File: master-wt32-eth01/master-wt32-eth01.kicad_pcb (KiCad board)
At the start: 2 copper layers, 61 x 72.4 mm, 12 parts, among them J1 24V Field, J2 24V System, J3 Enable, J4 Screw_Terminal_01x03, J5 Conn_01x06_Female, J6 Conn_01x06_Female, SW1 SW_DIP_x03, U1 LM2596-Board, U2 WT32-ETH0-Board, U3 PC817

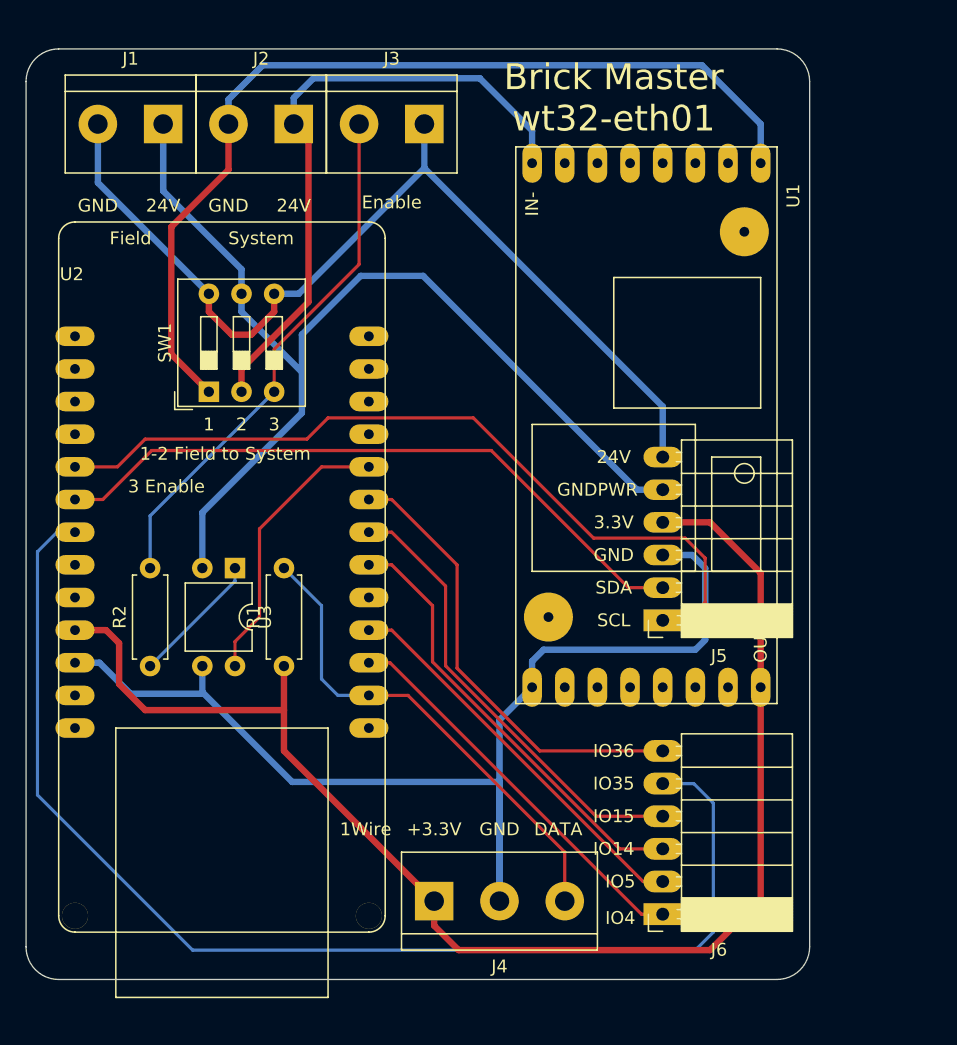
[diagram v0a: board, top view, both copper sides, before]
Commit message: v1.1
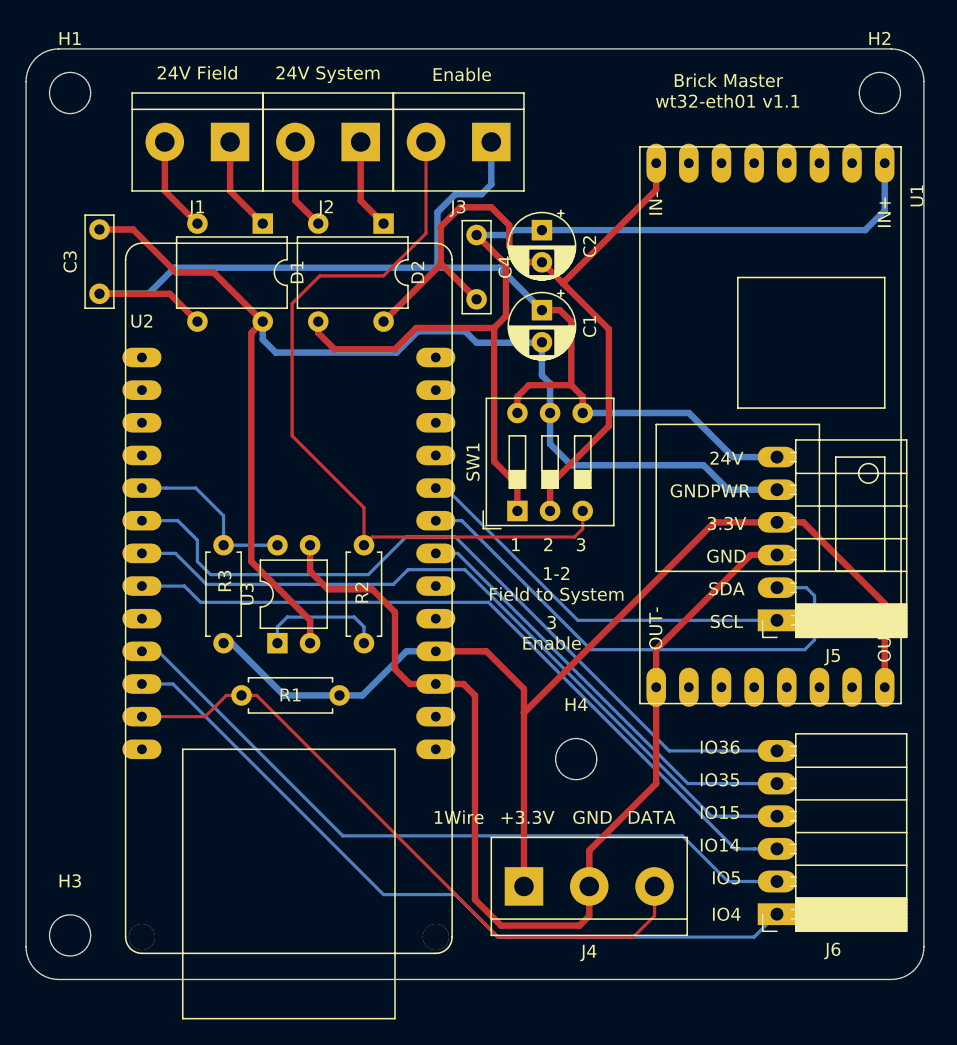
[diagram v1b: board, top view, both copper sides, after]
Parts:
- added C1: 1uF 50V, Capacitor_THT:CP_Radial_D5.0mm_P2.50mm, F.Cu at (103.6, 74.9)
- added C2: 1uF 50V, Capacitor_THT:CP_Radial_D5.0mm_P2.50mm, F.Cu at (103.6, 68.7)
- added C3: 100nF 63V, Capacitor_THT:C_Rect_L7.0mm_W2.0mm_P5.00mm, F.Cu at (69.2, 73.7)
- added C4: 100nF 63V, Capacitor_THT:C_Rect_L7.0mm_W2.0mm_P5.00mm, F.Cu at (98.6, 69.1)
- added D1: DB107, custom:DB107, F.Cu at (81.9, 68.2)
- added D2: DB107, custom:DB107, F.Cu at (91.3, 68.2)
- added H1: MountingHole, MountingHole:MountingHole_3.2mm_M3, F.Cu at (66.9, 58.0)
- added H2: MountingHole, MountingHole:MountingHole_3.2mm_M3, F.Cu at (129.9, 58.0)
- added H3: MountingHole, MountingHole:MountingHole_3.2mm_M3, F.Cu at (66.9, 123.6)
- added H4: MountingHole, MountingHole:MountingHole_3.2mm_M3, F.Cu at (106.3, 109.9)
- added R3: 100k, Resistor_THT:R_Axial_DIN0207_L6.3mm_D2.5mm_P7.62mm_Horizontal, F.Cu at (78.9, 100.8)
- U2: footprint boards:WT32-ETH0-Board -> boards:WT32-ETH01-Board-Reversed
- moved SW1 25.7 mm to (101.7, 90.6)
- moved R2 16.7 mm to (89.8, 100.8)
- moved U1 9.65 mm to (121.4, 83.8)
- moved J5 8.89 mm to (121.9, 99.1)
- moved J6 8.89 mm to (121.9, 121.9)
- moved J4 7.08 mm to (102.2, 119.8)
- moved U3 6.71 mm to (83.1, 100.8), turned to 90 degrees
- moved U2 5.46 mm to (83.9, 97.7)
- moved J1 5.39 mm to (79.4, 61.8)
- moved J2 5.39 mm to (89.5, 61.8)
- moved J3 5.39 mm to (99.7, 61.8)
- moved R1 4.89 mm to (87.9, 104.9), turned to 180 degrees
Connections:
- J1 pad 1: GNDPWR -> FIELD_IN-
- J1 pad 2: +24V -> FIELD_IN+
- J2 pad 1: Net-(J2-Pad1) -> SYSTEM_IN-
- J2 pad 2: Net-(J2-Pad2) -> SYSTEM_IN+
- SW1 pad 1: Net-(J2-Pad2) -> SYSTEM+
- SW1 pad 2: Net-(J2-Pad1) -> SYSTEM-
- U1 pad 1: Net-(J2-Pad2) -> SYSTEM+
- U1 pad 2: Net-(J2-Pad1) -> SYSTEM-
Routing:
- net SYSTEM+: track 0.00 -> 75.6 mm
- net Net-(J2-Pad2): track 73.2 -> 0.00 mm
- net GPIO35: track 95.2 -> 34.0 mm
- net SYSTEM-: track 0.00 -> 60.1 mm
- net Net-(J2-Pad1): track 48.9 -> 0.00 mm
- net SCL: track 62.4 -> 30.8 mm
- net GPIO4: track 31.0 -> 58.3 mm
- net GPIO5: track 31.0 -> 56.8 mm
- net GPIO36: track 35.7 -> 60.2 mm
- net GPIO14: track 34.6 -> 57.9 mm
- net GPIO15: track 35.6 -> 58.8 mm
- net +3V3: track 108.2 -> 86.4 mm
- net Net-(J3-Pad2): track 41.3 -> 59.8 mm
- net +24V: track 75.5 -> 90.3 mm
- net 1WIRE: track 38.2 -> 51.3 mm
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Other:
- board size 61 x 72.4 mm -> 69.9 x 72.4 mm
- board text added: "24V Field"
- board text added: "24V System"
- board text added: "Brick Master wt32-eth01 v1.1"
- board text removed: "Brick Master wt32-eth01"
- board text removed: "Field"
- board text removed: "System"
